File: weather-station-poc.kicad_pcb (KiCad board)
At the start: 4 copper layers, 155 x 88 mm, 135 parts, among them IC1 632723100011, IC2 TCPP01-M12, IC3 USBLC6-2SC6, IC4 BME690, IC5 S2-LPQTR, IC6 BALF-SPI2-01D3, IC7 STSAFA110S8OCD03, J1 Conn_ARM_JTAG_SWD_10, J2 61300311121, J3 61300311121, J4 61300511121, J5 61300311121, J6 687140149022, J7 687110183622, Q1 STL11N3LLH6, U1 STM32U5G9ZJTxQ, U2 BME280, U3 BMP581, Y1 NX2016SA-16MHZ-EXS00A-CS07826, Y2 NX2012SA-32.768K-STD-MUB-1, Y3 NX1612SA-50M-EXS00A-CS08403

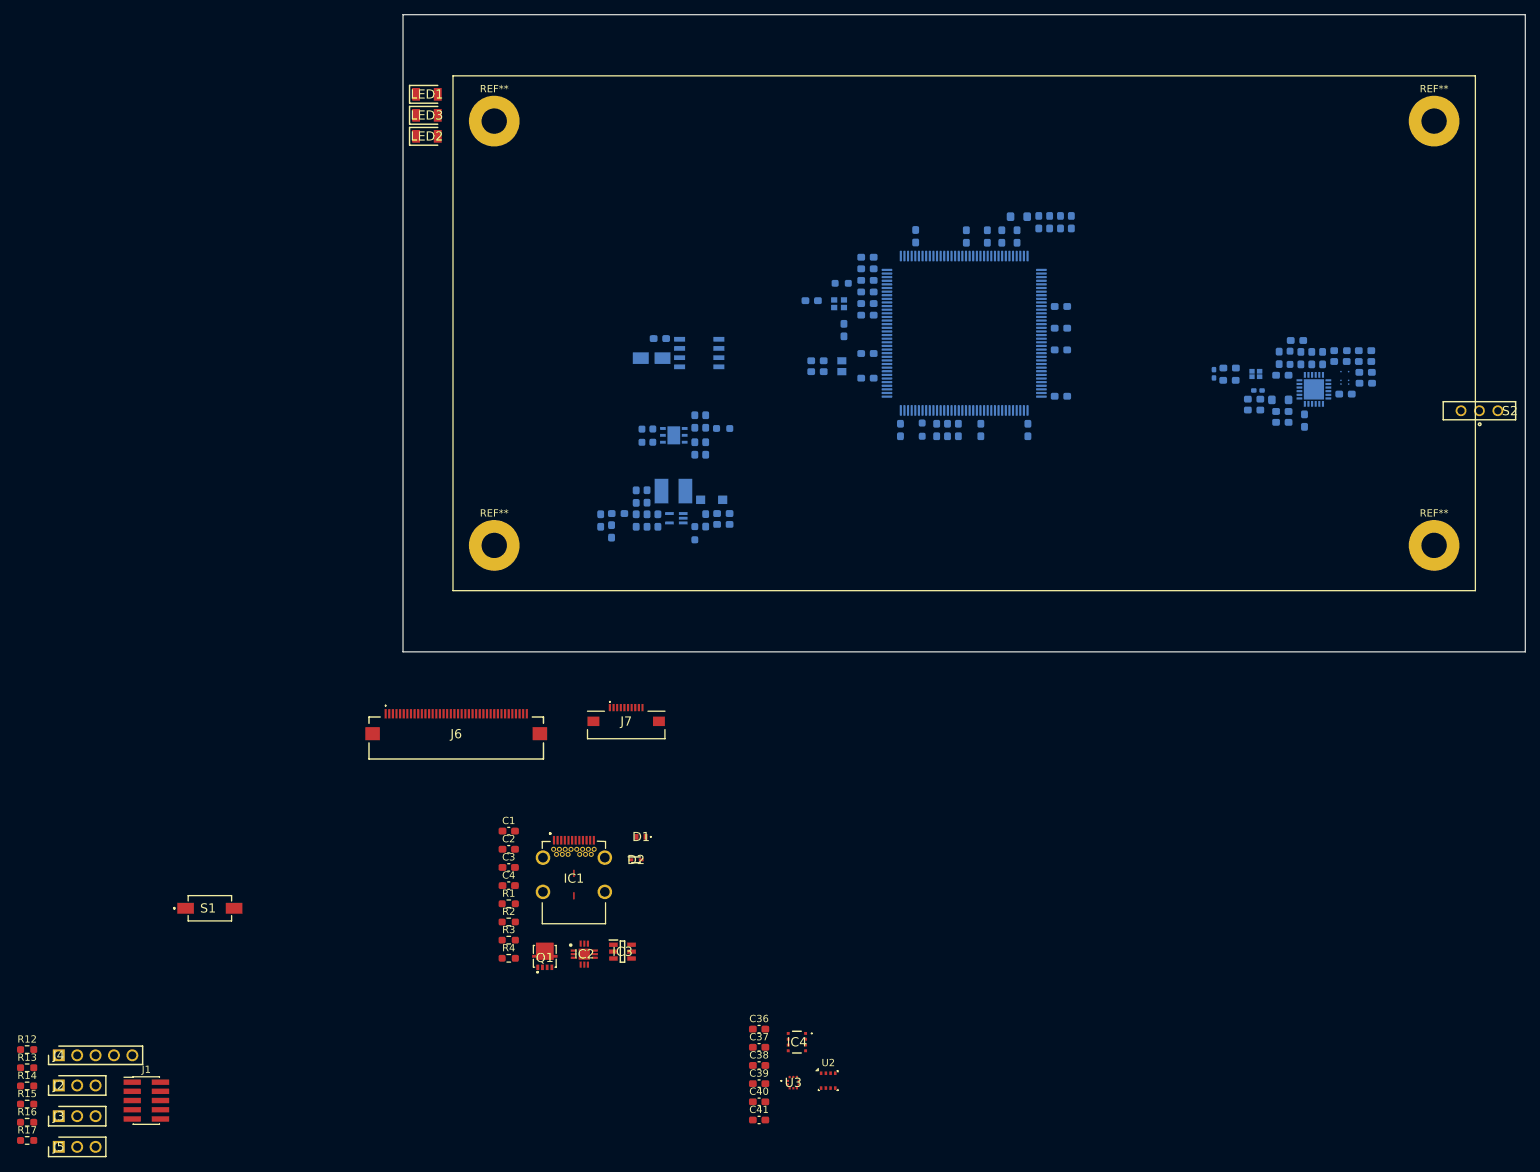
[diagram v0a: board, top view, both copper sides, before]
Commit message: Update weather-station-poc.kicad_pcb
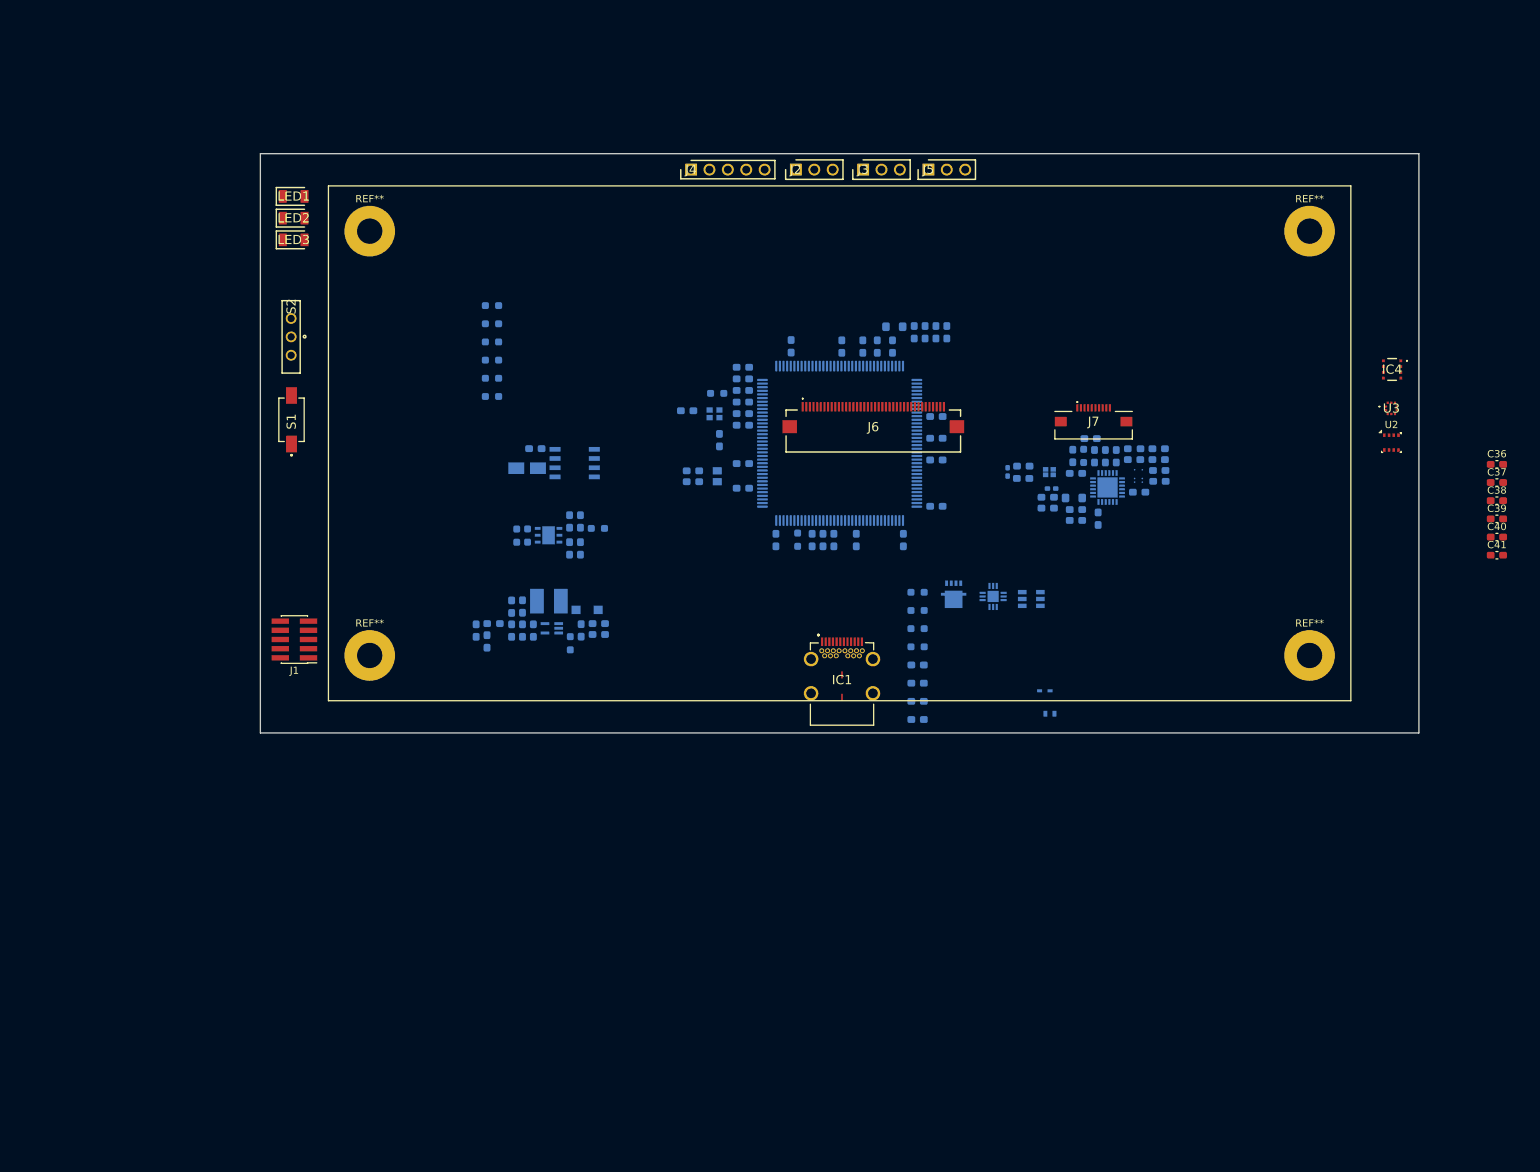
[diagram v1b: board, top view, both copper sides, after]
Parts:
- C1, C2, C3, C4, D1, D2, IC2, IC3, Q1, R1, R12, R13, R14, R15, R16, R17, R2, R3, R4: moved to B.Cu
- moved J5 180.7 mm to (158.0, 53.7)
- moved J3 171.5 mm to (148.9, 53.7)
- moved J2 162.4 mm to (139.7, 53.7)
- moved S2 160.4 mm to (72.0, 78.8), turned to -90 degrees
- moved J4 150.3 mm to (125.2, 53.7)
- moved R17 132.0 mm to (97.7, 72.5)
- moved C36 128.3 mm to (236.5, 94.4)
- moved C37 128.3 mm to (236.5, 96.9)
- moved C38 128.3 mm to (236.5, 99.4)
- moved C39 128.3 mm to (236.5, 101.9)
- moved C40 128.3 mm to (236.5, 104.4)
- moved C41 128.3 mm to (236.5, 107.0)
- moved R16 127.6 mm to (97.7, 75.0)
- moved U3 124.5 mm to (221.9, 86.7)
- moved IC4 124.0 mm to (222.0, 81.3)
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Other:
- board size 155 x 88 mm -> 160 x 80 mm
